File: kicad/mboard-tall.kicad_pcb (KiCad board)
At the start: 2 copper layers, 50.8 x 26.4 mm, 16 parts

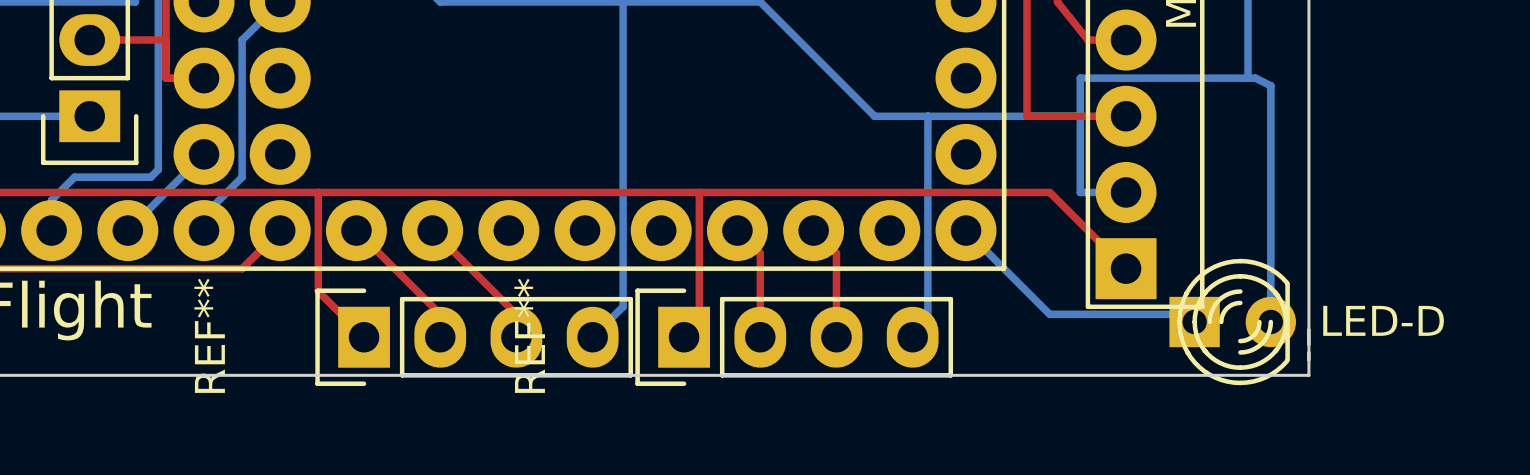
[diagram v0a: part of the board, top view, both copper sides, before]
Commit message: size tweaks
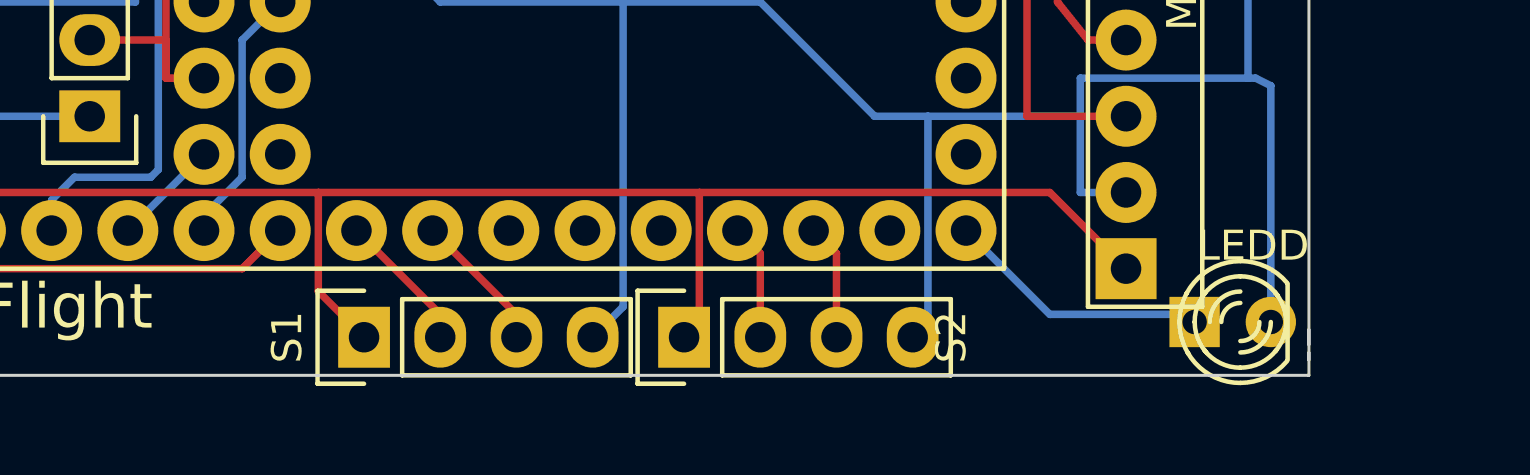
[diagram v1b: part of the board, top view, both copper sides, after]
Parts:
- REF: renamed from REF**; value LED-D -> LEDD
- S1: renamed from REF**; value Pin_Header_Straight_1x04 -> (none)
- renumbered REF** to S2
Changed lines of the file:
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@@
     (links 0)
     (no_connects 0)
-    (area 21.914524 32.403 76.157191 59.965001)
+    (area 21.914524 32.403 75.823953 61.411001)
     (thickness 1.6)
     (drawings 14)
@@
     (34 B.Paste user hide)
     (35 F.Paste user hide)
-    (36 B.SilkS user hide)
+    (36 B.SilkS user)
     (37 F.SilkS user)
     (38 B.Mask user hide)
@@
     (descr "LED 3mm - Lead pitch 100mil (2,54mm)")
     (tags "LED led 3mm 3MM 100mil 2,54mm")
-    (fp_text reference REF** (at 1.778 -2.794) (layer F.SilkS) hide
-      (effects (font (size 1 1) (thickness 0.15)))
-    )
-    (fp_text value LED-D (at 5 0) (layer F.SilkS)
+    (fp_text reference REF (at 1.778 -2.794) (layer F.SilkS) hide
+      (effects (font (size 1 1) (thickness 0.15)))
+    )
+    (fp_text value LEDD (at 0.682 -2.54) (layer F.SilkS)
       (effects (font (size 1 1) (thickness 0.15)))
     )
@@
     (descr "Through hole pin header")
     (tags "pin header")
-    (fp_text reference REF** (at 0 -5.1 90) (layer F.SilkS)
-      (effects (font (size 1 1) (thickness 0.15)))
-    )
-    (fp_text value Pin_Header_Straight_1x04 (at 0 -3.1 90) (layer F.Fab)
+    (fp_text reference S1 (at 0 -2.56 90) (layer F.SilkS)
+      (effects (font (size 1 1) (thickness 0.15)))
+    )
+    (fp_text value "" (at 0 -3.1 90) (layer F.Fab) hide
       (effects (font (size 1 1) (thickness 0.15)))
     )
@@
     (descr "Through hole pin header")
     (tags "pin header")
-    (fp_text reference REF** (at 0 -5.1 90) (layer F.SilkS)
-      (effects (font (size 1 1) (thickness 0.15)))
-    )
-    (fp_text value Pin_Header_Straight_1x04 (at 0 -3.1 90) (layer F.Fab)
+    (fp_text reference S2 (at 0 8.91 90) (layer F.SilkS)
+      (effects (font (size 1 1) (thickness 0.15)))
+    )
+    (fp_text value Pin_Header_Straight_1x04 (at 0 -3.1 90) (layer F.Fab) hide
       (effects (font (size 1 1) (thickness 0.15)))
     )
@@
   (gr_line (start 74.93 34.29) (end 74.93 59.69) (angle 90) (layer Edge.Cuts) (width 0.1))
   (gr_line (start 24.13 34.29) (end 74.93 34.29) (angle 90) (layer Edge.Cuts) (width 0.1))
-  (segment (start 59.182 59.436) (end 59.182 56.642) (width 0.25) (layer F.Cu) (net 0) (status 400000))
-  (segment (start 59.182 56.642) (end 58.42 55.88) (width 0.25) (layer F.Cu) (net 0) (status 800000))
-  (segment (start 56.642 59.436) (end 56.642 56.642) (width 0.25) (layer F.Cu) (net 0) (status 400000))
-  (segment (start 56.642 56.642) (end 55.88 55.88) (width 0.25) (layer F.Cu) (net 0) (status 800000))
-  (segment (start 62.23 52.07) (end 62.23 58.928) (width 0.25) (layer B.Cu) (net 0) (status 800000))
-  (segment (start 62.23 58.928) (end 61.722 59.436) (width 0.25) (layer B.Cu) (net 0) (status C00000))
-  (segment (start 54.61 54.61) (end 54.61 58.928) (width 0.25) (layer F.Cu) (net 0) (status 800000))
-  (segment (start 54.61 58.928) (end 54.102 59.436) (width 0.25) (layer F.Cu) (net 0) (status C00000))
+  (segment (start 59.182 59.436) (end 59.182 56.642) (width 0.25) (layer F.Cu) (net 0))
+  (segment (start 59.182 56.642) (end 58.42 55.88) (width 0.25) (layer F.Cu) (net 0))
+  (segment (start 56.642 59.436) (end 56.642 56.642) (width 0.25) (layer F.Cu) (net 0))
+  (segment (start 56.642 56.642) (end 55.88 55.88) (width 0.25) (layer F.Cu) (net 0))
+  (segment (start 62.23 52.07) (end 62.23 58.928) (width 0.25) (layer B.Cu) (net 0))
+  (segment (start 62.23 58.928) (end 61.722 59.436) (width 0.25) (layer B.Cu) (net 0))
+  (segment (start 54.61 54.61) (end 54.61 58.928) (width 0.25) (layer F.Cu) (net 0))
+  (segment (start 54.61 58.928) (end 54.102 59.436) (width 0.25) (layer F.Cu) (net 0))
   (segment (start 48.514 59.436) (end 48.514 58.674) (width 0.25) (layer F.Cu) (net 0))
   (segment (start 48.514 58.674) (end 45.72 55.88) (width 0.25) (layer F.Cu) (net 0))
